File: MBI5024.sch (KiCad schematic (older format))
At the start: 3 parts, among them J1 Conn_01x12, J2 Conn_01x12, U1 MBI5024

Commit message: Change project name to MBI5024
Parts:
- U1: symbol MBI5024_Symbol_Library:MBI5024 -> MBI5024:MBI5024
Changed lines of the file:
@@
 $EndDescr
 $Comp
-L MBI5024_Symbol_Library:MBI5024 U1
+L MBI5024:MBI5024 U1
 U 1 1 5C293359
 P 5500 3600

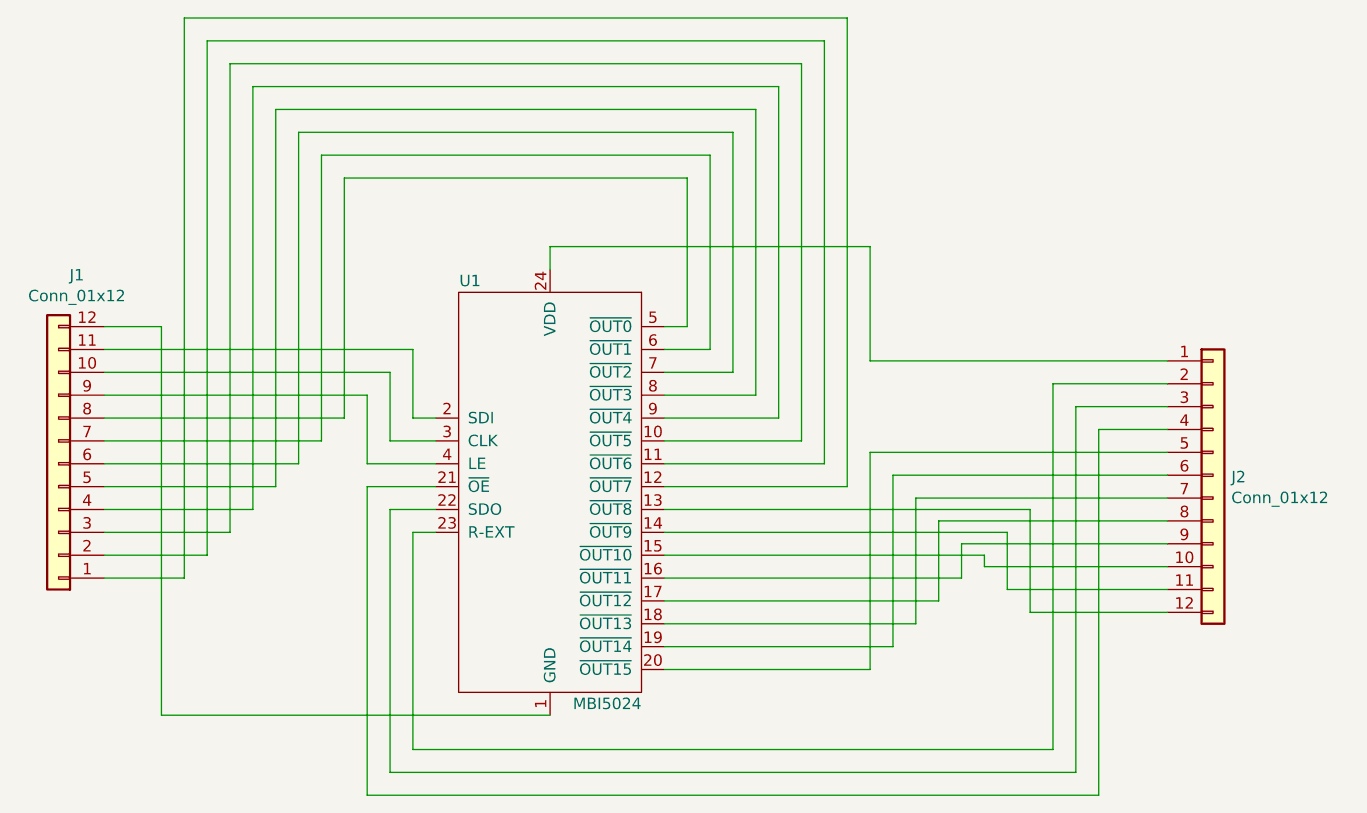
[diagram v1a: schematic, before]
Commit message: Fix up schematic for the adapter
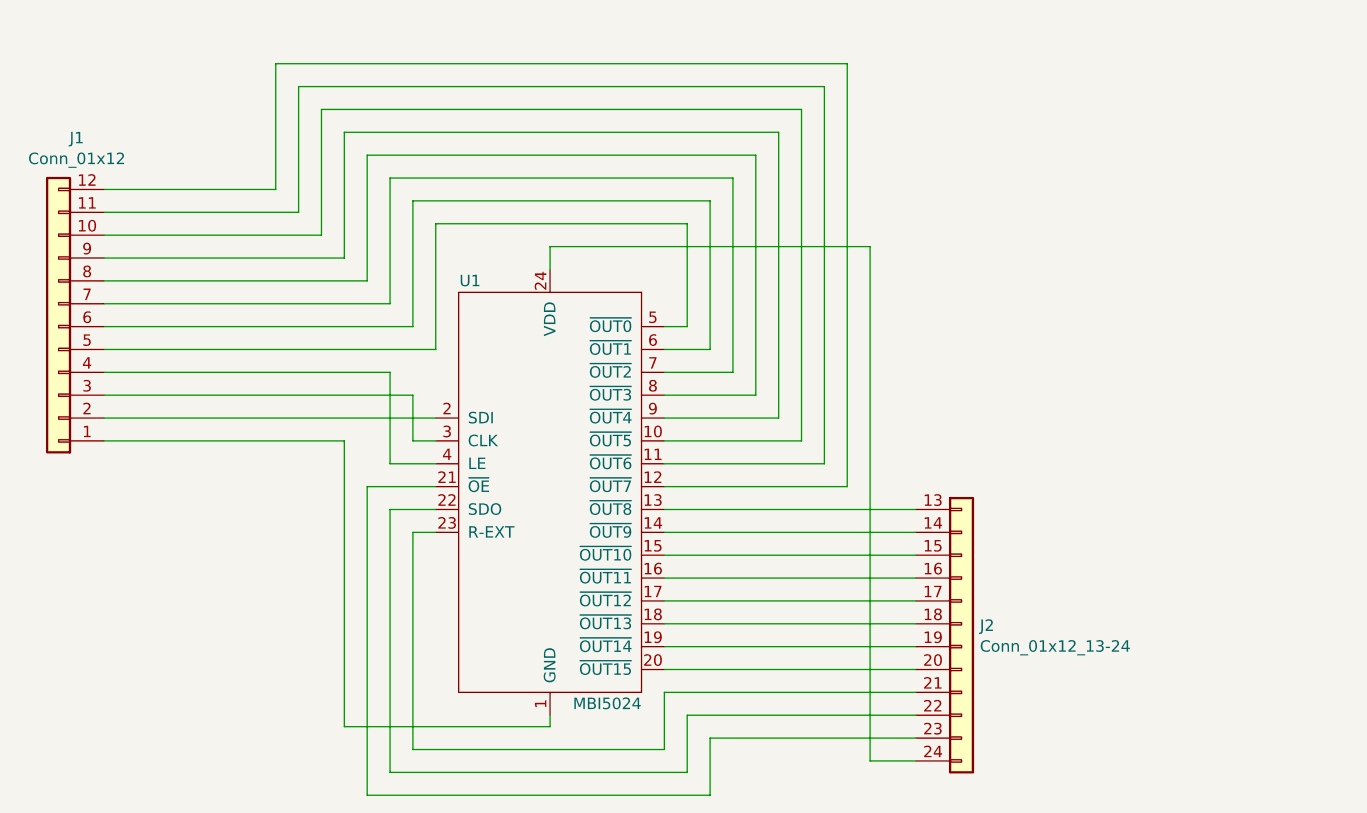
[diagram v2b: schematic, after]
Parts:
- removed J2: Conn_01x12, Connector_PinHeader_2.54mm:PinHeader_1x12_P2.54mm_Vertical, symbol Connector_Generic:Conn_01x12
- added J2: Conn_01x12_13-24, symbol conn_01x12_13-24:Conn_01x12_13-24
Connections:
- net at U1.1 (GND): now also J1.1 (Pin_1); no longer J1.12 (Pin_12)
- net at U1.10 (~OUT5): now also J1.10 (Pin_10); no longer J1.3 (Pin_3)
- net at U1.11 (~OUT6): now also J1.11 (Pin_11); no longer J1.2 (Pin_2)
- net at U1.12 (~OUT7): now also J1.12 (Pin_12); no longer J1.1 (Pin_1)
- net at U1.13 (~OUT8): now also J2.13 (Pin_1)
- net at U1.14 (~OUT9): now also J2.14 (Pin_2)
- net at U1.15 (~OUT10): now also J2.15 (Pin_3)
- net at U1.16 (~OUT11): now also J2.16 (Pin_4)
- net at U1.17 (~OUT12): now also J2.17 (Pin_5)
- net at U1.18 (~OUT13): now also J2.18 (Pin_6)
- net at U1.19 (~OUT14): now also J2.19 (Pin_7)
- net at U1.2 (SDI): now also J1.2 (Pin_2); no longer J1.11 (Pin_11)
- net at U1.20 (~OUT15): now also J2.20 (Pin_8)
- net at U1.21 (~OE): now also J2.23 (Pin_11)
- net at U1.22 (SDO): now also J2.22 (Pin_10)
- net at U1.23 (R-EXT): now also J2.21 (Pin_9)
- net at U1.24 (VDD): now also J2.24 (Pin_12)
- net at U1.3 (CLK): now also J1.3 (Pin_3); no longer J1.10 (Pin_10)
- net at U1.4 (LE): now also J1.4 (Pin_4); no longer J1.9 (Pin_9)
- net at U1.5 (~OUT0): now also J1.5 (Pin_5); no longer J1.8 (Pin_8)
- net at U1.6 (~OUT1): now also J1.6 (Pin_6); no longer J1.7 (Pin_7)
- net at U1.7 (~OUT2): now also J1.7 (Pin_7); no longer J1.6 (Pin_6)
- net at U1.8 (~OUT3): now also J1.8 (Pin_8); no longer J1.5 (Pin_5)
- net at U1.9 (~OUT4): now also J1.9 (Pin_9); no longer J1.4 (Pin_4)
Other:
- moved on the sheet: J1
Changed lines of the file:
@@
 EESchema Schematic File Version 4
+LIBS:MBI5024-cache
 EELAYER 26 0
 EELAYER END
@@
 L Connector_Generic:Conn_01x12 J1
 U 1 1 5C29369A
-P 3350 3550
-F 0 "J1" H 3270 2725 50  0000 C CNN
-F 1 "Conn_01x12" H 3270 2816 50  0000 C CNN
-F 2 "Connector_PinHeader_2.54mm:PinHeader_1x12_P2.54mm_Vertical" H 3350 3550 50  0001 C CNN
-F 3 "~" H 3350 3550 50  0001 C CNN
-	1    3350 3550
+P 3350 2950
+F 0 "J1" H 3270 2125 50  0000 C CNN
+F 1 "Conn_01x12" H 3270 2216 50  0000 C CNN
+F 2 "Connector_PinHeader_2.54mm:PinHeader_1x12_P2.54mm_Vertical" H 3350 2950 50  0001 C CNN
+F 3 "~" H 3350 2950 50  0001 C CNN
+	1    3350 2950
 	-1   0    0    1
 $EndComp
+Wire Wire Line
+	6000 3150 6300 3150
+Wire Wire Line
+	6000 3250 6400 3250
+Wire Wire Line
+	6000 3350 6500 3350
+Wire Wire Line
+	6000 3450 6600 3450
+Wire Wire Line
+	6000 3550 6700 3550
+Wire Wire Line
+	6000 3650 6800 3650
+Wire Wire Line
+	6000 2950 6100 2950
+Wire Wire Line
+	6000 3050 6200 3050
+Wire Wire Line
+	5000 3850 4900 3850
+Wire Wire Line
+	4900 3850 4900 4800
+Wire Wire Line
+	4900 4800 6000 4800
+Wire Wire Line
+	5000 3750 4800 3750
+Wire Wire Line
+	4800 3750 4800 4900
+Wire Wire Line
+	4800 4900 6100 4900
+Wire Wire Line
+	5000 3650 4700 3650
+Wire Wire Line
+	4700 3650 4700 5000
+Wire Wire Line
+	6900 2600 5500 2600
+Wire Wire Line
+	5500 2600 5500 2700
+Wire Wire Line
+	4700 5000 6200 5000
 $Comp
-L Connector_Generic:Conn_01x12 J2
-U 1 1 5C2936F4
-P 8400 3600
-F 0 "J2" H 8480 3592 50  0000 L CNN
-F 1 "Conn_01x12" H 8480 3501 50  0000 L CNN
-F 2 "Connector_PinHeader_2.54mm:PinHeader_1x12_P2.54mm_Vertical" H 8400 3600 50  0001 C CNN
-F 3 "~" H 8400 3600 50  0001 C CNN
-	1    8400 3600
+L conn_01x12_13-24:Conn_01x12_13-24 J2
+U 1 1 5C458646
+P 7300 4250
+F 0 "J2" H 7380 4242 50  0000 L CNN
+F 1 "Conn_01x12_13-24" H 7380 4151 50  0000 L CNN
+F 2 "" H 7300 4250 50  0001 C CNN
+F 3 "~" H 7300 4250 50  0001 C CNN
+	1    7300 4250
 	1    0    0    -1
 $EndComp
 Wire Wire Line
-	5000 3350 4900 3350
-Wire Wire Line
-	5000 3450 4800 3450
-Wire Wire Line
-	5000 3550 4700 3550
-Wire Wire Line
-	6000 3150 6300 3150
-Wire Wire Line
-	6000 3250 6400 3250
-Wire Wire Line
-	6000 3350 6500 3350
-Wire Wire Line
-	6000 3450 6600 3450
-Wire Wire Line
-	6000 3550 6700 3550
-Wire Wire Line
-	6000 3650 6800 3650
-Wire Wire Line
-	5500 4650 3800 4650
-Wire Wire Line
-	6000 4350 7000 4350
+	6000 4800 6000 4550
+Wire Wire Line
+	6100 4900 6100 4650
+Wire Wire Line
+	6200 5000 6200 4750
+Wire Wire Line
+	6900 2600 6900 4850
+Wire Wire Line
+	6900 4850 7100 4850
+Wire Wire Line
+	6200 4750 7100 4750
+Wire Wire Line
+	6100 4650 7100 4650
+Wire Wire Line
+	6000 4550 7100 4550
+Wire Wire Line
+	6000 4450 7100 4450
+Wire Wire Line
+	6000 4350 7100 4350
 Wire Wire Line
 	6000 4250 7100 4250
 Wire Wire Line
-	6000 4150 7200 4150
-Wire Wire Line
-	6000 4050 7300 4050
-Wire Wire Line
-	6000 3950 7400 3950
-Wire Wire Line
-	6000 3850 7500 3850
-Wire Wire Line
-	6000 2950 6100 2950
-Wire Wire Line
-	6100 2950 6100 2300
-Wire Wire Line
-	6100 2300 4600 2300
-Wire Wire Line
-	6000 3050 6200 3050
-Wire Wire Line
-	6200 3050 6200 2200
-Wire Wire Line
-	6200 2200 4500 2200
-Wire Wire Line
-	6300 3150 6300 2100
-Wire Wire Line
-	6300 2100 4400 2100
-Wire Wire Line
-	6400 3250 6400 2000
-Wire Wire Line
-	6500 3350 6500 1900
-Wire Wire Line
-	6400 2000 4300 2000
-Wire Wire Line
-	6500 1900 4200 1900
-Wire Wire Line
-	6600 3450 6600 1800
-Wire Wire Line
-	6600 1800 4100 1800
-Wire Wire Line
-	6700 3550 6700 1700
-Wire Wire Line
-	6700 1700 4000 1700
-Wire Wire Line
-	6800 3650 6800 1600
-Wire Wire Line
-	6800 1600 3900 1600
-Wire Wire Line
-	6900 4450 6900 3500
-Wire Wire Line
-	6900 4450 6000 4450
-Wire Wire Line
-	7000 4350 7000 3600
-Wire Wire Line
-	7100 4250 7100 3700
-Wire Wire Line
-	7200 4150 7200 3800
-Wire Wire Line
-	7300 4050 7300 3900
-Wire Wire Line
-	7400 3950 7400 4000
-Wire Wire Line
-	7500 3850 7500 4100
-Wire Wire Line
-	6000 3750 7600 3750
-Wire Wire Line
-	7600 3750 7600 4200
-Wire Wire Line
-	5000 3850 4900 3850
-Wire Wire Line
-	4900 3850 4900 4800
-Wire Wire Line
-	4900 4800 7700 4800
-Wire Wire Line
-	7700 4800 7700 3200
-Wire Wire Line
-	5000 3750 4800 3750
-Wire Wire Line
-	4800 3750 4800 4900
-Wire Wire Line
-	4800 4900 7800 4900
-Wire Wire Line
-	7800 4900 7800 3300
-Wire Wire Line
-	6900 3500 8200 3500
-Wire Wire Line
-	7000 3600 8200 3600
-Wire Wire Line
-	7100 3700 8200 3700
-Wire Wire Line
-	7200 3800 8200 3800
-Wire Wire Line
-	7300 3900 8200 3900
-Wire Wire Line
-	7400 4000 8200 4000
-Wire Wire Line
-	7500 4100 8200 4100
-Wire Wire Line
-	7600 4200 8200 4200
-Wire Wire Line
-	5000 3650 4700 3650
-Wire Wire Line
-	4700 3650 4700 5000
-Wire Wire Line
-	4700 5000 7900 5000
-Wire Wire Line
-	7900 5000 7900 3400
-Wire Wire Line
-	7900 3400 8200 3400
-Wire Wire Line
-	7800 3300 8200 3300
-Wire Wire Line
-	7700 3200 8200 3200
-Wire Wire Line
-	8200 3100 6900 3100
-Wire Wire Line
-	6900 3100 6900 2600
-Wire Wire Line
-	6900 2600 5500 2600
-Wire Wire Line
-	5500 2600 5500 2700
-Wire Wire Line
-	4900 3350 4900 3050
-Wire Wire Line
-	3550 3050 4900 3050
-Wire Wire Line
-	4800 3450 4800 3150
-Wire Wire Line
-	3550 3150 4800 3150
-Wire Wire Line
-	4700 3550 4700 3250
-Wire Wire Line
-	3550 3250 4700 3250
-Wire Wire Line
-	4600 3350 4600 2300
-Wire Wire Line
-	3550 3350 4600 3350
-Wire Wire Line
-	4500 3450 4500 2200
-Wire Wire Line
-	3550 3450 4500 3450
-Wire Wire Line
-	4400 3550 4400 2100
-Wire Wire Line
-	3550 3550 4400 3550
-Wire Wire Line
-	4300 3650 4300 2000
-Wire Wire Line
-	3550 3650 4300 3650
-Wire Wire Line
-	4200 3750 4200 1900
-Wire Wire Line
-	3550 3750 4200 3750
-Wire Wire Line
-	4100 3850 4100 1800
-Wire Wire Line
-	3550 3850 4100 3850
-Wire Wire Line
-	4000 3950 4000 1700
-Wire Wire Line
-	3550 3950 4000 3950
-Wire Wire Line
-	3900 4050 3900 1600
-Wire Wire Line
-	3550 4050 3900 4050
-Wire Wire Line
-	3800 2950 3800 4650
-Wire Wire Line
-	3550 2950 3800 2950
+	6000 4150 7100 4150
+Wire Wire Line
+	6000 4050 7100 4050
+Wire Wire Line
+	6000 3950 7100 3950
+Wire Wire Line
+	6000 3850 7100 3850
+Wire Wire Line
+	6000 3750 7100 3750
+Wire Wire Line
+	6100 2950 6100 2500
+Wire Wire Line
+	6100 2500 5000 2500
+Wire Wire Line
+	6200 3050 6200 2400
+Wire Wire Line
+	6200 2400 4900 2400
+Wire Wire Line
+	6300 3150 6300 2300
+Wire Wire Line
+	6300 2300 4800 2300
+Wire Wire Line
+	6400 3250 6400 2200
+Wire Wire Line
+	6400 2200 4700 2200
+Wire Wire Line
+	6500 3350 6500 2100
+Wire Wire Line
+	6500 2100 4600 2100
+Wire Wire Line
+	6600 3450 6600 2000
+Wire Wire Line
+	6600 2000 4500 2000
+Wire Wire Line
+	6700 3550 6700 1900
+Wire Wire Line
+	6700 1900 4400 1900
+Wire Wire Line
+	6800 3650 6800 1800
+Wire Wire Line
+	6800 1800 4300 1800
+Wire Wire Line
+	5000 3350 3550 3350
+Wire Wire Line
+	5000 3450 4900 3450
+Wire Wire Line
+	4900 3450 4900 3250
+Wire Wire Line
+	4900 3250 3550 3250
+Wire Wire Line
+	5000 3550 4800 3550
+Wire Wire Line
+	4800 3550 4800 3150
+Wire Wire Line
+	4800 3150 3550 3150
+Wire Wire Line
+	5500 4650 5500 4700
+Wire Wire Line
+	5500 4700 4600 4700
+Wire Wire Line
+	4600 4700 4600 3450
+Wire Wire Line
+	4600 3450 3550 3450
+Wire Wire Line
+	3550 3050 5000 3050
+Wire Wire Line
+	5000 3050 5000 2500
+Wire Wire Line
+	3550 2950 4900 2950
+Wire Wire Line
+	4900 2950 4900 2400
+Wire Wire Line
+	3550 2850 4800 2850
+Wire Wire Line
+	4800 2850 4800 2300
+Wire Wire Line
+	3550 2750 4700 2750
+Wire Wire Line
+	4700 2750 4700 2200
+Wire Wire Line
+	3550 2650 4600 2650
+Wire Wire Line
+	4600 2650 4600 2100
+Wire Wire Line
+	3550 2550 4500 2550
+Wire Wire Line
+	4500 2550 4500 2000
+Wire Wire Line
+	3550 2450 4400 2450
+Wire Wire Line
+	4400 2450 4400 1900
+Wire Wire Line
+	3550 2350 4300 2350
+Wire Wire Line
+	4300 2350 4300 1800
 $EndSCHEMATC
